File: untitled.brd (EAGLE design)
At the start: 59.4 x 57.8 mm, 25 parts, among them IC1 REG1117F

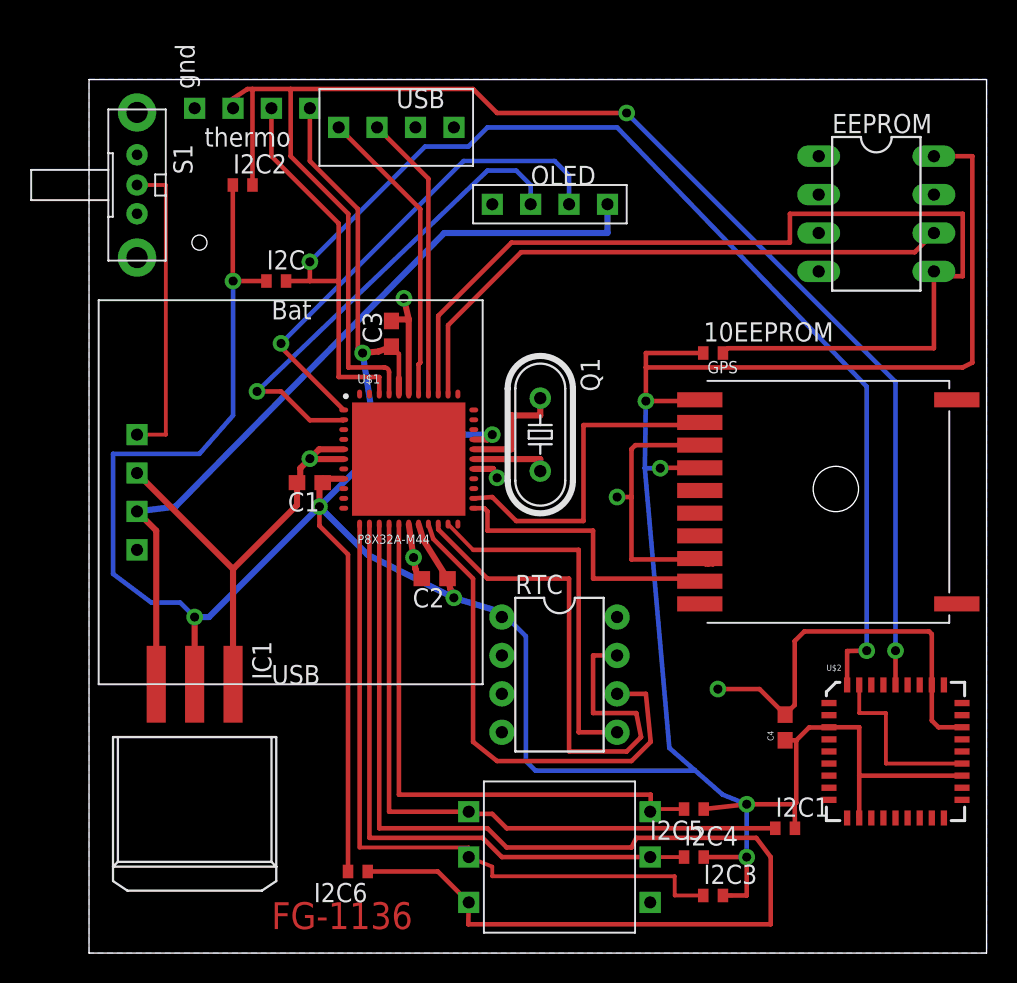
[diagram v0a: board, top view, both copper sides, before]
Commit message: DRC cleanup
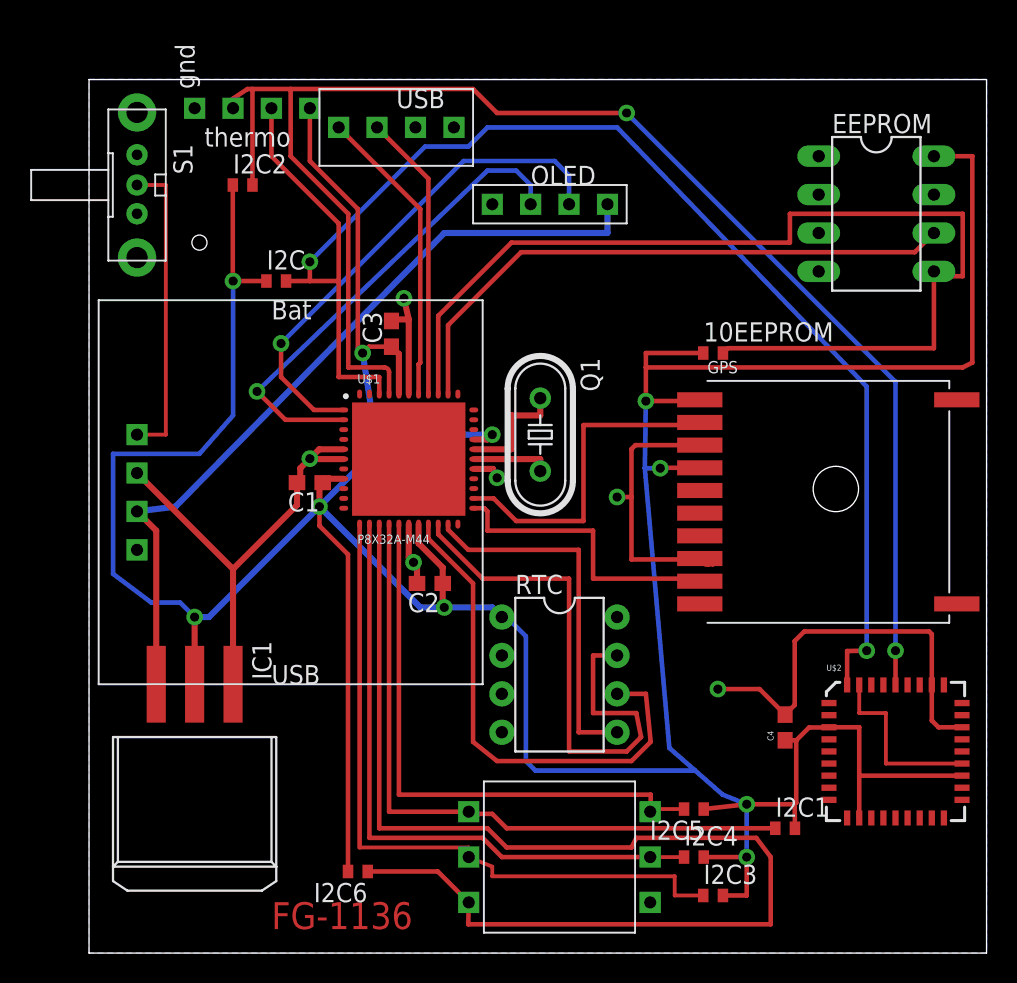
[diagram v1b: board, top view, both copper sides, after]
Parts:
- moved C2 0.45 mm to (56.2, 34.6)
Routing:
- net +3V3: track 292.2 -> 293.7 mm
- net N$11: track 32.5 -> 33.6 mm
- net N$16: track 0.64 -> 0.00 mm
- net GND: track 91.3 -> 92.0 mm
